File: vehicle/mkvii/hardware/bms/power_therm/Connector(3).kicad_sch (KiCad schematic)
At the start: 1 part

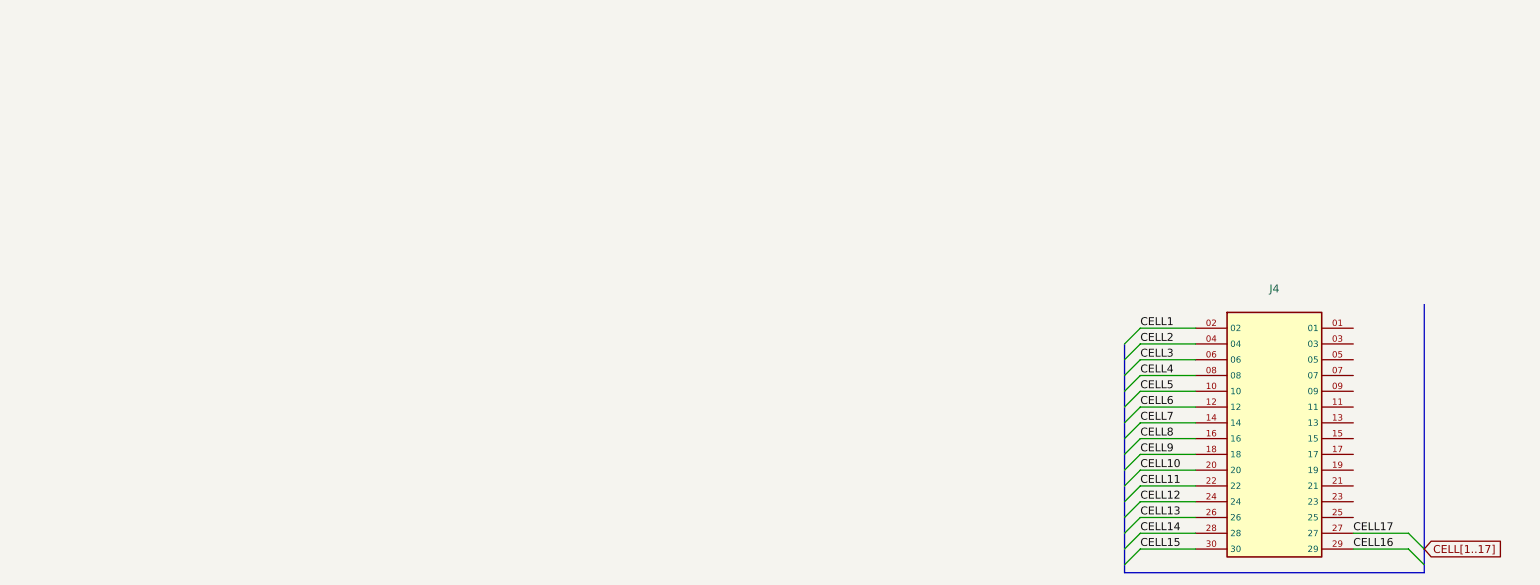
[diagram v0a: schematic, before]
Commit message: final draft pre leads revisions)
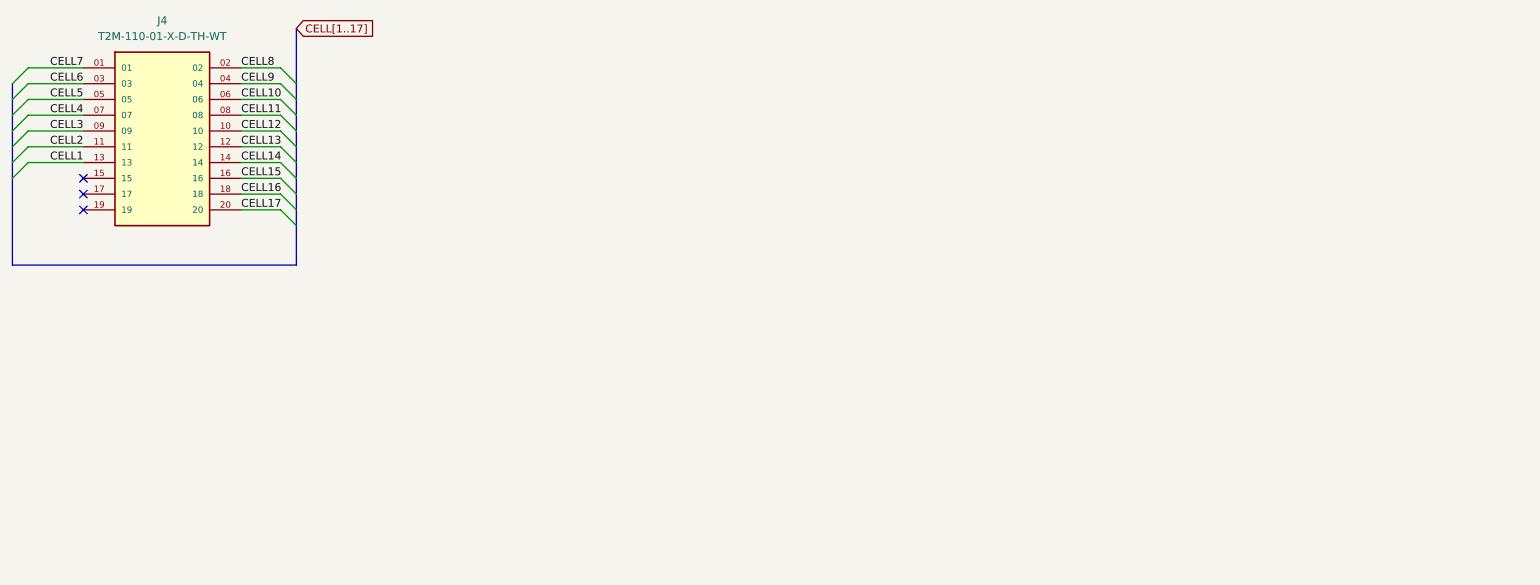
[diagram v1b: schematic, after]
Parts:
- removed J4: ~, oem:Samtec 20, symbol formula:Samtec_30_pin
- added J4: T2M-110-01-X-D-TH-WT, OEM:SAMTEC_T2M-110-01-X-D-TH-WT, symbol oem:CONN_T2M_20P
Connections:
- net CELL1: now also J4.13
- net CELL10: now also J4.06
- net CELL11: now also J4.08
- net CELL12: now also J4.10
- net CELL13: now also J4.12
- net CELL14: now also J4.14
- net CELL15: now also J4.16
- net CELL16: now also J4.18
- net CELL17: now also J4.20
- net CELL2: now also J4.11
- net CELL3: now also J4.09
- net CELL4: now also J4.07
- net CELL5: now also J4.05
- net CELL6: now also J4.03
- net CELL7: now also J4.01
- net CELL8: now also J4.02
- net CELL9: now also J4.04
- no-connect marks 0 -> 3
